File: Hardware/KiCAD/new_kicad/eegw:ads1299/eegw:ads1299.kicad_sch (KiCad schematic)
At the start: 30 parts, among them J1 ESP32_R2, J11 ESP32_L, J2 gpioADS, J3 ESP32_Left, J5 ESP32_Right, J7 ESP32_R1, J9 ESP32_R3, U1 ADS1299IPAG

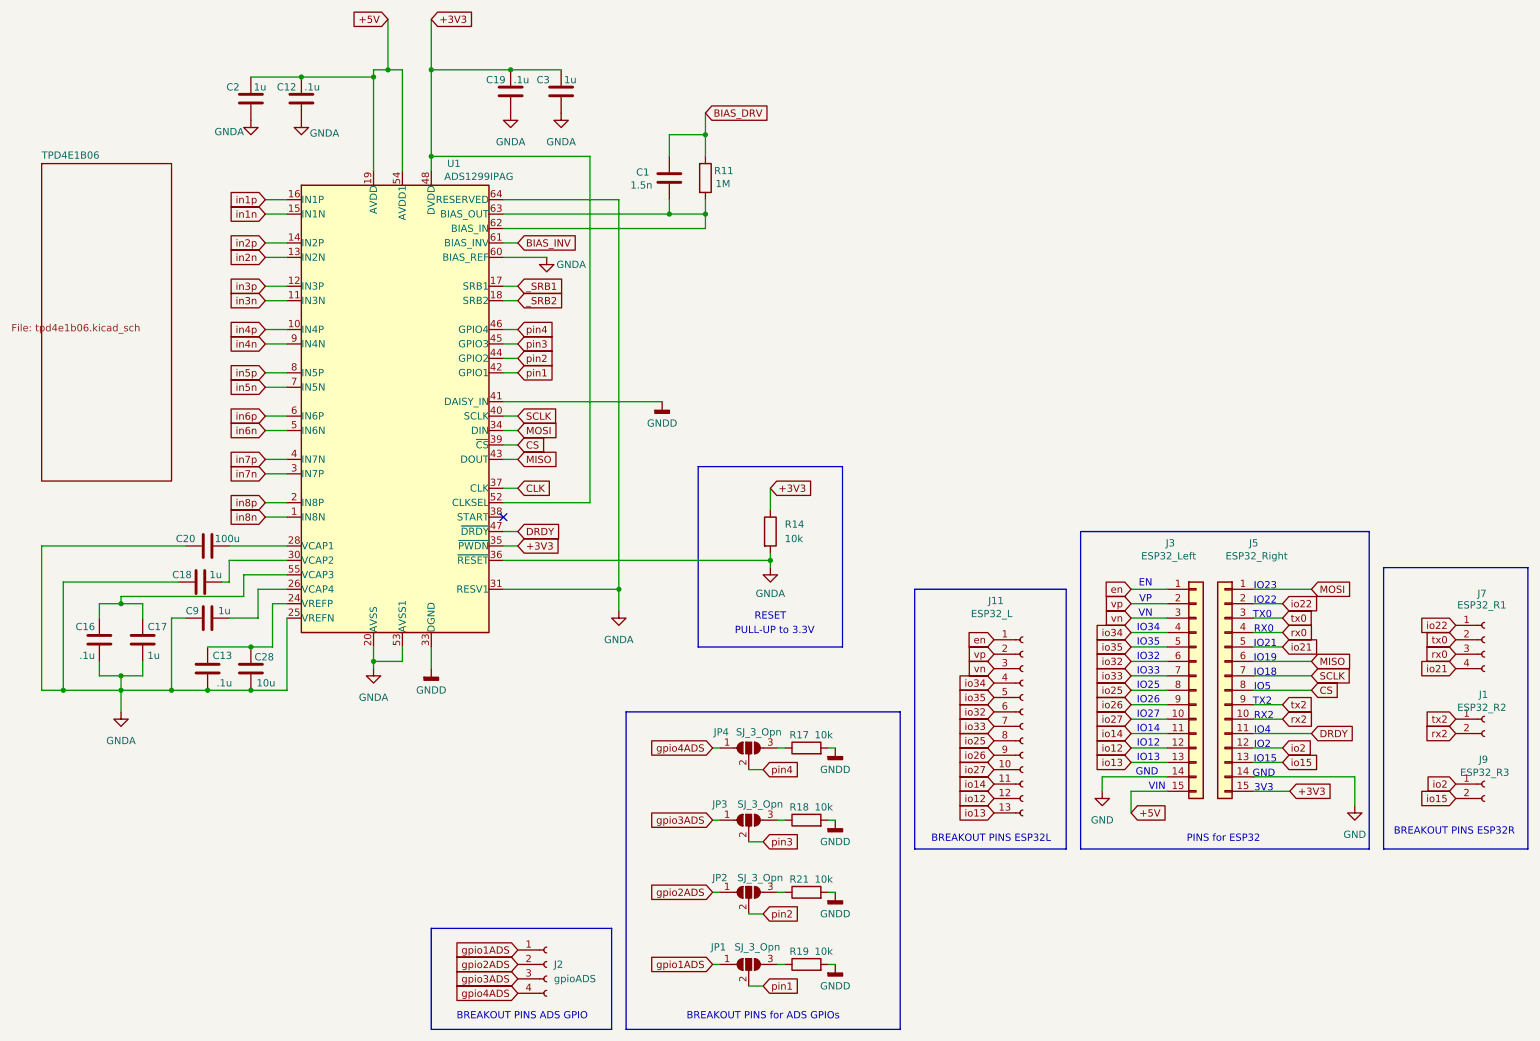
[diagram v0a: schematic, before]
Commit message: update filled zone & geograpgically annotated pcb
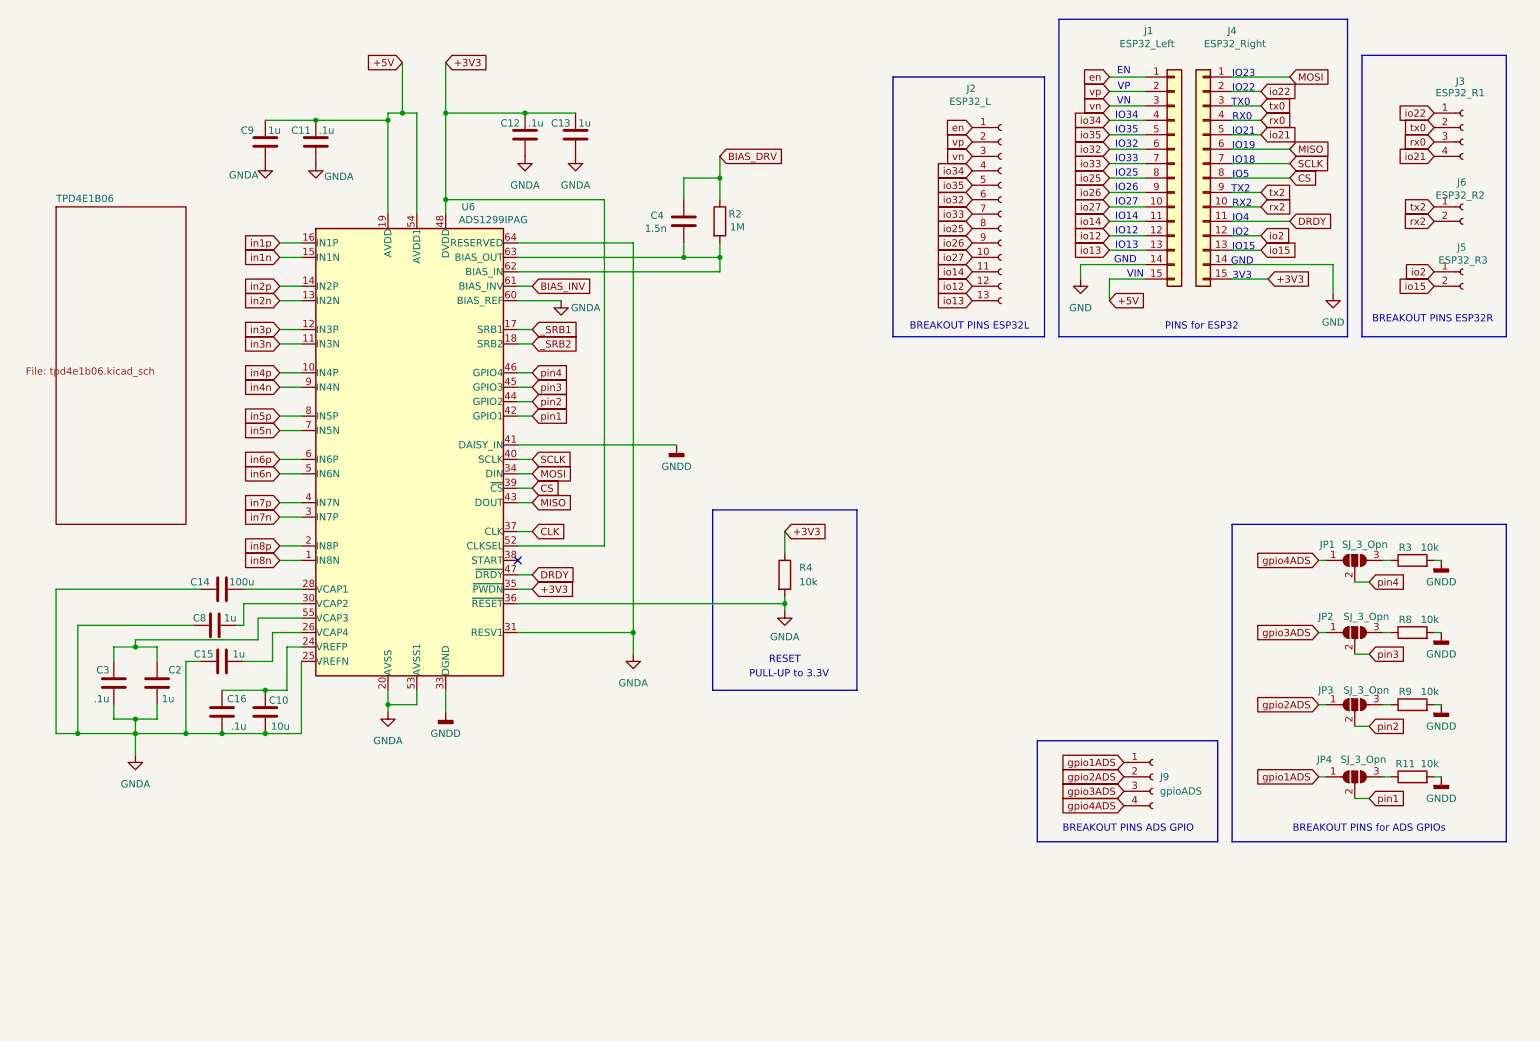
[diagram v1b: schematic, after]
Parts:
- renumbered C28 to C10, C12 to C11, C19 to C12, C3 to C13, C20 to C14, C9 to C15, C13 to C16, C17 to C2, C16 to C3, C1 to C4, C18 to C8, C2 to C9, J3 to J1, J11 to J2, J7 to J3, J5 to J4, J9 to J5, J1 to J6, J2 to J9, JP4 to JP1, JP3 to JP2, JP2 to JP3, JP1 to JP4, R19 to R11, R11 to R2, R17 to R3, R14 to R4, R18 to R8, R21 to R9, U1 to U6
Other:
- moved on the sheet: C10, C11, C12, C13, C14, C15, C16, C2, C3, C4, C8, C9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
